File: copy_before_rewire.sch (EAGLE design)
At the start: 62 parts, among them Q1 500mA, Q2 500mA, Q3 500mA, U1 HX711, U2 HX711, U3 5V, U4 STM32F0XXC1T, U5 PCF8574T/3,512SOT162-1-M, U6 HX711, U7 3.3V/150mA

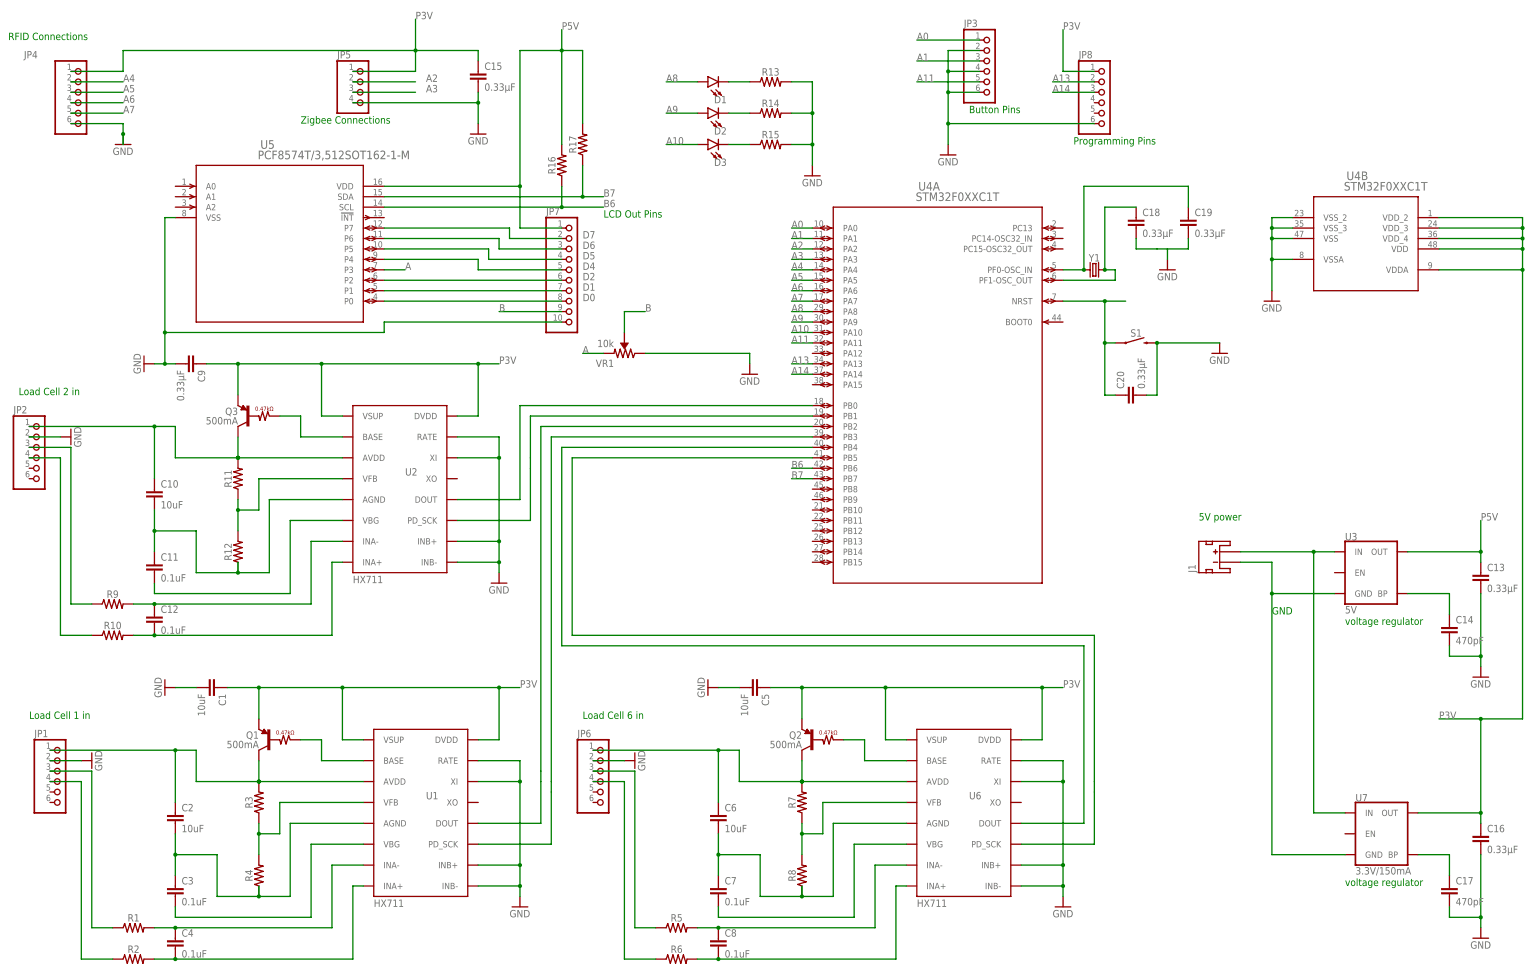
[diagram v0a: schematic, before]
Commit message: final stuff
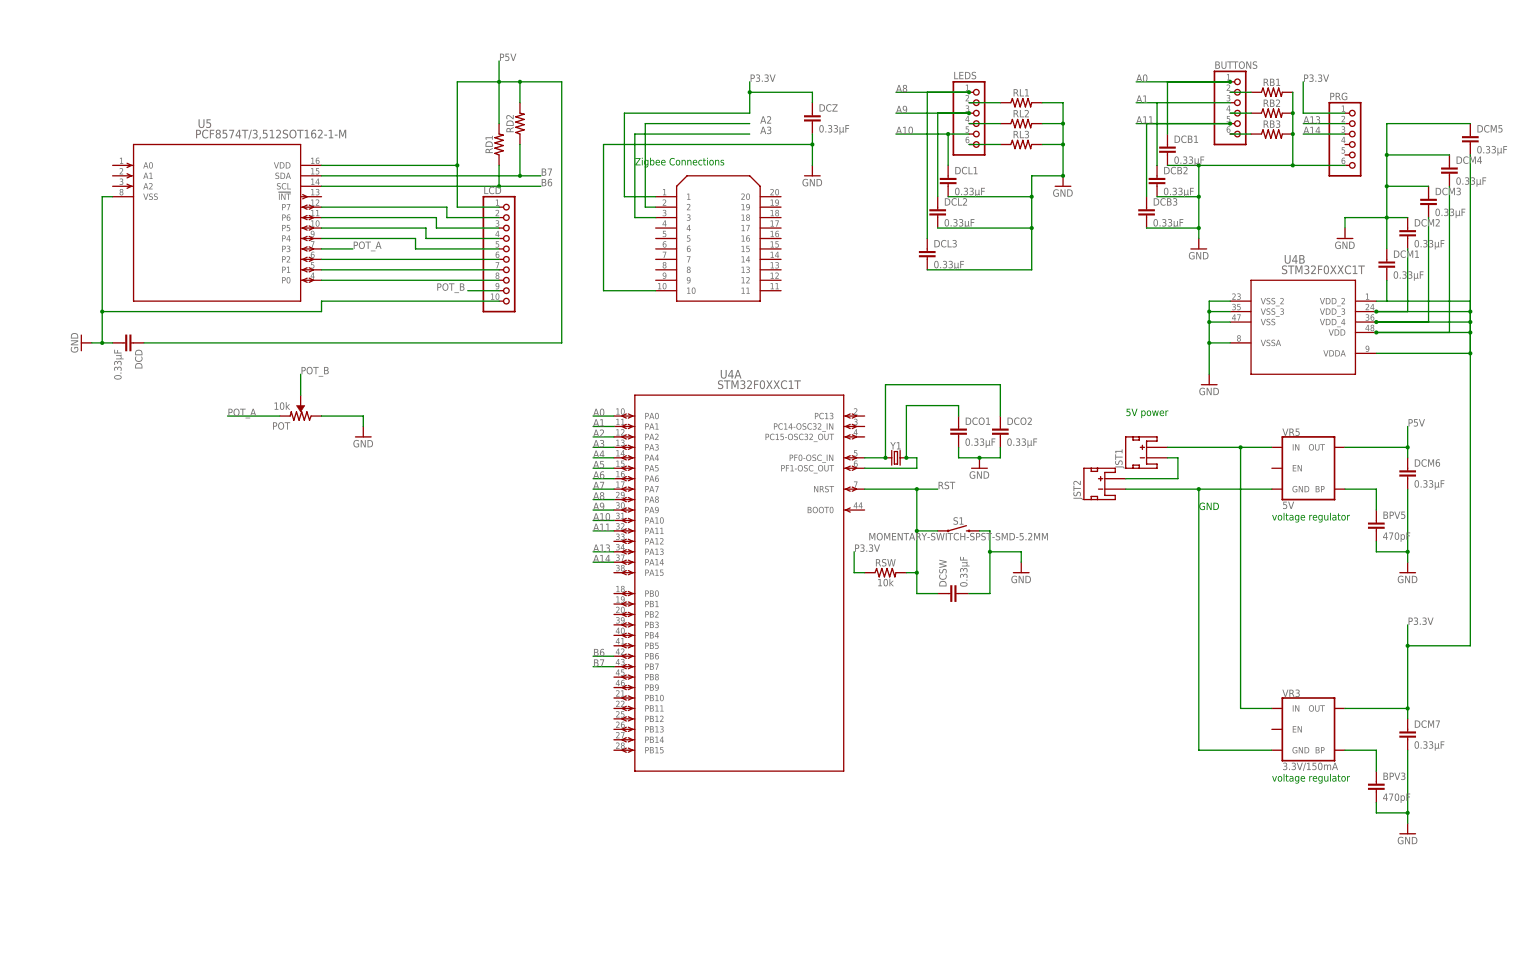
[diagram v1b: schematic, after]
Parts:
- removed C1, C10, C2, C5, C6: 10uF, SparkFun-Capacitors:10UF-0603-6.3V-20%
- removed C11, C12, C3, C4, C7, C8: 0.1uF, SparkFun-Capacitors:0.1UF-0603-25V-(+80/-20%)
- removed C13, C15, C16, C18, C19, C20, C9: 0.33µF, SparkFun-Capacitors:0.33UF/330NF-0805-50V-10%
- removed C14, C17: 470pF, SparkFun-Capacitors:470PF-0603-50V-5%
- removed D1, D2, D3: (no value), SparkFun-LED:LED5MM
- removed J1: (no value), SparkFun-Connectors:JST_2MM_MALE
- removed JP1, JP2, JP3, JP4, JP6, JP8: (no value), pinhead:PINHD-1X6
- removed JP5: (no value), pinhead:PINHD-1X4
- removed JP7: (no value), pinhead:PINHD-1X10
- removed Q1, Q2, Q3: 500mA, SparkFun-DiscreteSemi:TRANS_PNP_RES-DDTB142TC
- removed R1, R10, R11, R12, R13, R14, R15, R16, R17, R2, R3, R4, R5, R6, R7, R8, R9: (no value), SparkFun-Resistors:RESISTOR0603
- removed U1, U2, U6: HX711, SparkFun-IC-Conversion:HX711
- removed U3: 5V, SparkFun-IC-Power:V_REG_MIC52055V
- removed U7: 3.3V/150mA, SparkFun-IC-Power:V_REG_MIC52053.3V
- removed VR1: 10k, SparkFun-Resistors:TRIMPOT-PTH-10MM-KNOB-1/2W-10%
- added BPV3, BPV5: 470pF, SparkFun-Capacitors:470PF-0603-50V-5%
- added BUTTONS, LEDS, PRG: (no value), pinhead:PINHD-1X6
- added DCB1, DCB2, DCB3, DCD, DCL1, DCL2, DCL3, DCM1, DCM2, DCM3, DCM4, DCM5, DCM6, DCM7, DCO1, DCO2, DCSW, DCZ: 0.33µF, SparkFun-Capacitors:0.33UF/330NF-0805-50V-10%
- added JST1, JST2: (no value), SparkFun-Connectors:JST_2MM_MALE
- added LCD: (no value), pinhead:PINHD-1X10
- added POT: 10k, SparkFun-Resistors:TRIMPOT-PTH-10MM-KNOB-1/2W-10%
- added RB1, RB2, RB3, RD1, RD2, RL1, RL2, RL3: (no value), SparkFun-Resistors:RESISTOR0805
- added RSW: 10k, SparkFun-Resistors:10KOHM-0603-1/10W-1%
- added U$1: XB24-BPIT-004, XB24-BPIT-004:XB24-BPIT-004
- added VR3: 3.3V/150mA, SparkFun-IC-Power:V_REG_MIC52053.3V
- added VR5: 5V, SparkFun-IC-Power:V_REG_MIC52055V
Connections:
- removed net A: U5.P3, VR1.CCW
- removed net B: JP7.9, VR1.WIPER
- removed net D0: JP7.8, U5.P0
- removed net D1: JP7.7, U5.P1
- removed net D2: JP7.6, U5.P2
- removed net D4: JP7.5, U5.P4
- removed net D5: JP7.4, U5.P5
- removed net D6: JP7.3, U5.P6
- removed net D7: JP7.2, U5.P7
- removed net N$13: JP6.4, R6.1
- removed net N$17: C6.1, JP6.1, Q2.C, R7.2, U6.AVDD
- removed net N$18: C6.2, C7.1, R8.1, U6.AGND
- removed net N$19: R7.1, R8.2, U6.VFB
- removed net N$20: C7.2, U6.VBG
- removed net N$23: JP2.3, R9.1
- removed net N$24: JP2.4, R10.1
- removed net N$25: C12.1, R9.2, U2.INA-
- removed net N$26: C12.2, R10.2, U2.INA+
- removed net N$27: Q3.B, U2.BASE
- removed net N$28: C10.1, JP2.1, Q3.C, R11.2, U2.AVDD
- removed net N$29: C10.2, C11.1, R12.1, U2.AGND
- removed net N$30: R11.1, R12.2, U2.VFB
- removed net N$31: C11.2, U2.VBG
- removed net N$39: D1.C, R13.1
- removed net N$41: D2.C, R14.1
- removed net N$42: D3.C, R15.1
- removed net N$54: U4A.PB5, U6.PD_SCK
- removed net N$55: U4A.PB4, U6.DOUT
- removed net N$56: U1.PD_SCK, U4A.PB3
- removed net N$57: U1.DOUT, U4A.PB2
- removed net N$58: U2.PD_SCK, U4A.PB1
- removed net N$59: U2.DOUT, U4A.PB0
- removed net P3V: C1.1, C15.1, C16.1, C5.1, C9.1, JP4.1, JP5.1, JP8.1, Q1.E, Q2.E, Q3.E, U1.DVDD, U1.VSUP, U2.DVDD, U2.VSUP, U4B.VDD, U4B.VDDA, U4B.VDD_2, U4B.VDD_3, U4B.VDD_4, U6.DVDD, U6.VSUP, U7.OUT
- new net N$10: LCD.3, U5.P6
- new net P3.3V: DCM1.2, DCM2.2, DCM3.2, DCM4.2, DCM5.2, DCM7.1, DCZ.1, PRG.1, RSW.1, U$1.1, U4B.VDD, U4B.VDDA, U4B.VDD_2, U4B.VDD_3, U4B.VDD_4, VR3.OUT
- new net POT_A: POT.CCW, U5.P3
- new net POT_B: LCD.9, POT.WIPER
- new net RST: DCSW.1, RSW.2, S1.1, U4A.NRST
- net A0: now also BUTTONS.1, DCB1.1; no longer JP3.1
- net A1: now also BUTTONS.3; no longer JP3.3
- net A10: now also DCL1.1, LEDS.5; no longer D3.A
- net A11: now also BUTTONS.5, DCB3.1; no longer JP3.5
- net A13: now also PRG.2; no longer JP8.2
- net A14: now also PRG.3; no longer JP8.3
- net A2: now also U$1.2; no longer JP5.2
- net A3: now also U$1.3; no longer JP5.3
- net A4: no longer JP4.2
- net A5: no longer JP4.3
- net A6: no longer JP4.4
- net A7: no longer JP4.5
- net A8: now also DCL3.1, LEDS.1; no longer D1.A
- net A9: now also DCL2.1, LEDS.3; no longer D2.A
- net B6: now also RD1.1; no longer R16.1
- net B7: now also RD2.1; no longer R17.1
- net GND: now also BPV3.2, BPV5.2, DCB1.2, DCB2.2, DCB3.2, DCD.2, DCL1.2, DCL2.2, DCL3.2, DCM1.1, DCM2.1, DCM3.1, DCM4.1, DCM5.1, DCM6.2, DCM7.2, DCO1.2, DCO2.2, DCSW.2, DCZ.2, LCD.10, POT.CW, PRG.6, RB1.2, RB2.2, RB3.2, RL1.2, RL2.2, RL3.2, U$1.10; no longer C1.2, C13.2, C14.2, C15.2, C16.2, C17.2, C18.2, C19.2, C20.2, C5.2, C9.2, JP1.2, JP2.2, JP3.2, JP3.4, JP3.6, JP4.6, JP5.4, JP6.2, JP7.10, JP8.6, R13.2, R14.2, R15.2, U1.INB+, U1.INB-, U1.RATE, U1.XI, U2.INB+, U2.INB-, U2.RATE, U2.XI, U6.INB+, U6.INB-, U6.RATE, U6.XI, VR1.CW
- net N$1: now also JST1.-, JST2.+; no longer C20.1, S1.1, U4A.NRST
- net N$11: now also LCD.4, U5.P5; no longer C3.2, U1.VBG
- net N$12: now also LCD.5, U5.P4; no longer JP6.3, R5.1
- net N$14: now also LCD.6, U5.P2; no longer C8.1, R5.2, U6.INA-
- net N$15: now also LCD.7, U5.P1; no longer C8.2, R6.2, U6.INA+
- net N$16: now also LCD.8, U5.P0; no longer Q2.B, U6.BASE
- net N$2: now also BUTTONS.4, RB2.1; no longer JP1.3, R1.1
- net N$21: now also DCO2.1; no longer C19.1
- net N$22: now also DCO1.1; no longer C18.1
- net N$3: now also LEDS.6, RL3.1; no longer JP1.4, R2.1
- net N$32: now also JST2.-, VR3.GND, VR5.GND; no longer J1.-, U3.GND, U7.GND
- net N$34: now also BPV3.1, VR3.BP; no longer C17.1, U7.BP
- net N$37: now also BPV5.1, VR5.BP; no longer C14.1, U3.BP
- net N$38: now also JST1.+, VR3.IN, VR5.IN; no longer J1.+, U3.IN, U7.IN
- net N$4: now also LEDS.4, RL2.1; no longer C4.1, R1.2, U1.INA-
- net N$5: now also LEDS.2, RL1.1; no longer C4.2, R2.2, U1.INA+
- net N$6: now also BUTTONS.2, RB1.1; no longer Q1.B, U1.BASE
- net N$7: now also BUTTONS.6, RB3.1; no longer C2.1, JP1.1, Q1.C, R3.2, U1.AVDD
- net N$8: now also DCB2.1; no longer C2.2, C3.1, R4.1, U1.AGND
- net N$9: now also LCD.2, U5.P7; no longer R3.1, R4.2, U1.VFB
- net P5V: now also DCD.1, DCM6.1, LCD.1, RD1.2, RD2.2, VR5.OUT; no longer C13.1, JP7.1, R16.2, R17.2, U3.OUT
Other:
- note removed: "Button Pins"
- note removed: "LCD Out Pins"
- note removed: "Load Cell 1 in"
- note removed: "Load Cell 2 in"
- note removed: "Load Cell 6 in"
- note removed: "Programming Pins"
- note removed: "RFID Connections"
- moved on the sheet: S1, U4A, U4B, U5, Y1
